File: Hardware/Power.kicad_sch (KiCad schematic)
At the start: 63 parts

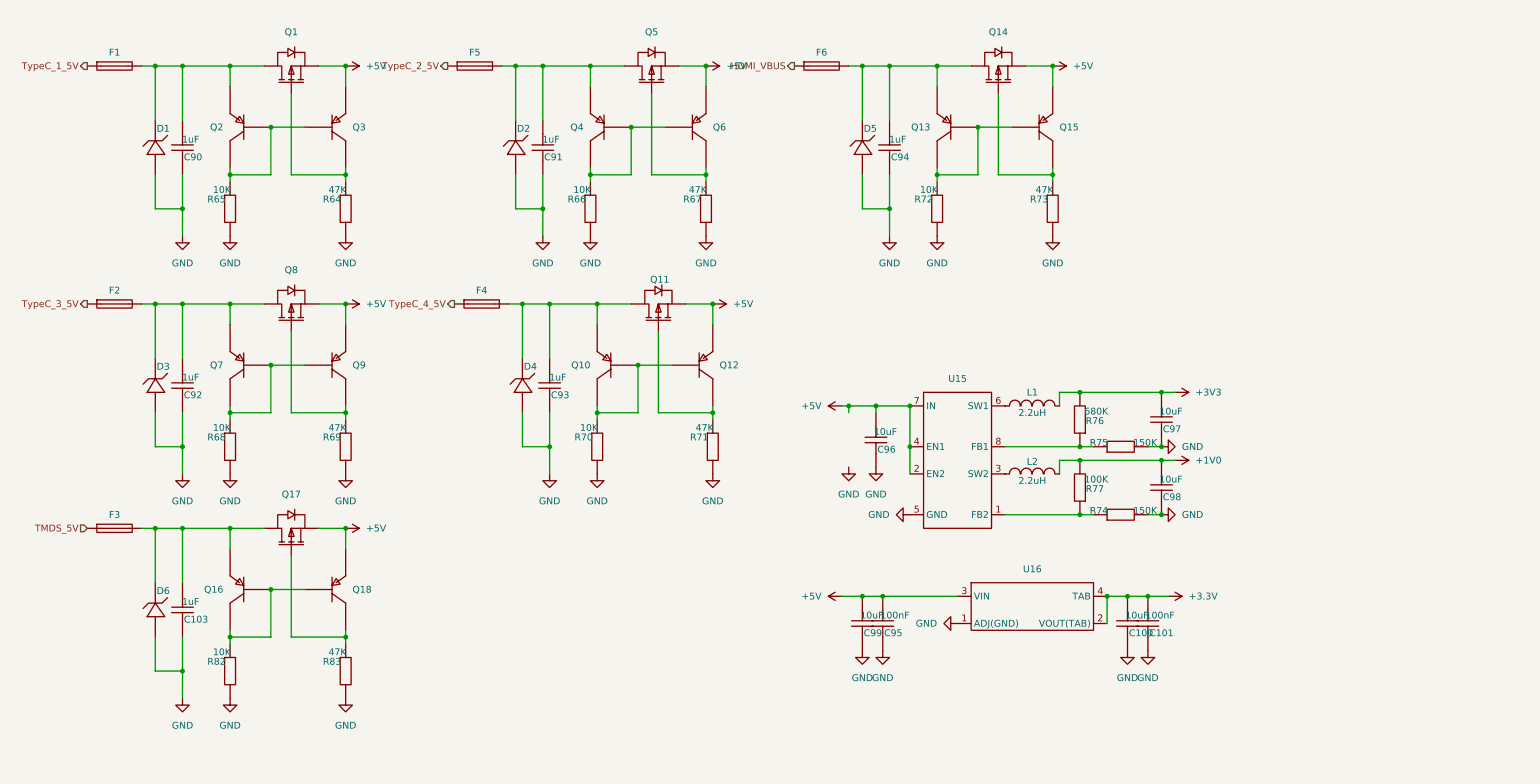
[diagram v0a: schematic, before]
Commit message: 开始PCB布局
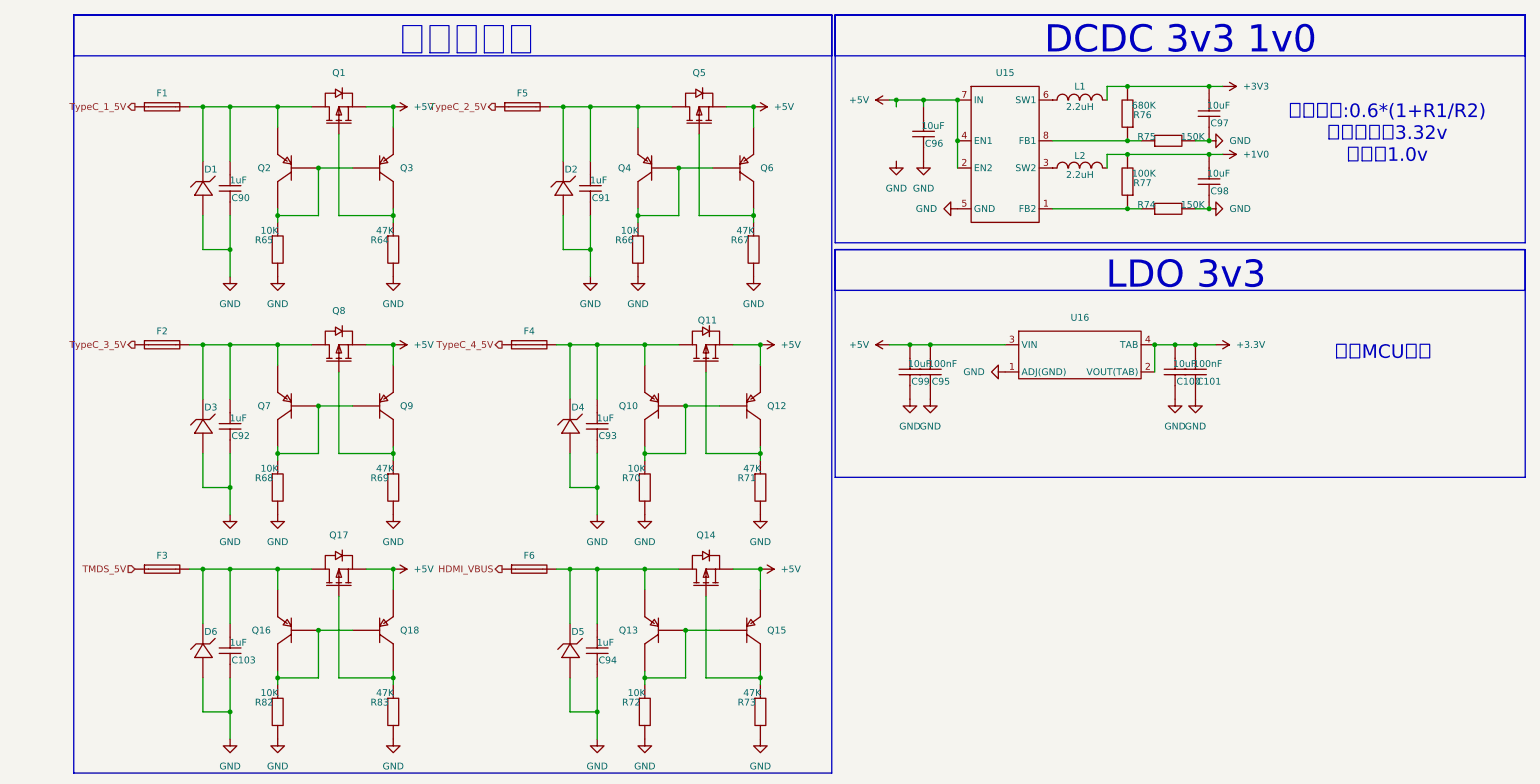
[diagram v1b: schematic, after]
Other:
- note added: "DCDC 3v3 1v0"
- note added: "LDO 3v3"
- note added: "计算公式:0.6*(1+R1/R2) 上路输出为3.32v 下路为1.0v"
- note added: "负责MCU供电"
- note added: "防浪涌电路"
- moved on the sheet: C100, C101, C103, C90, C91, C92, C93, C94, C95, C96, C97, C98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
